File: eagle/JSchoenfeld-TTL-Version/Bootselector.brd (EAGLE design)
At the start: 22 x 64.2 mm, 10 parts, among them IC3 74HC00N, IC4 74HC157N

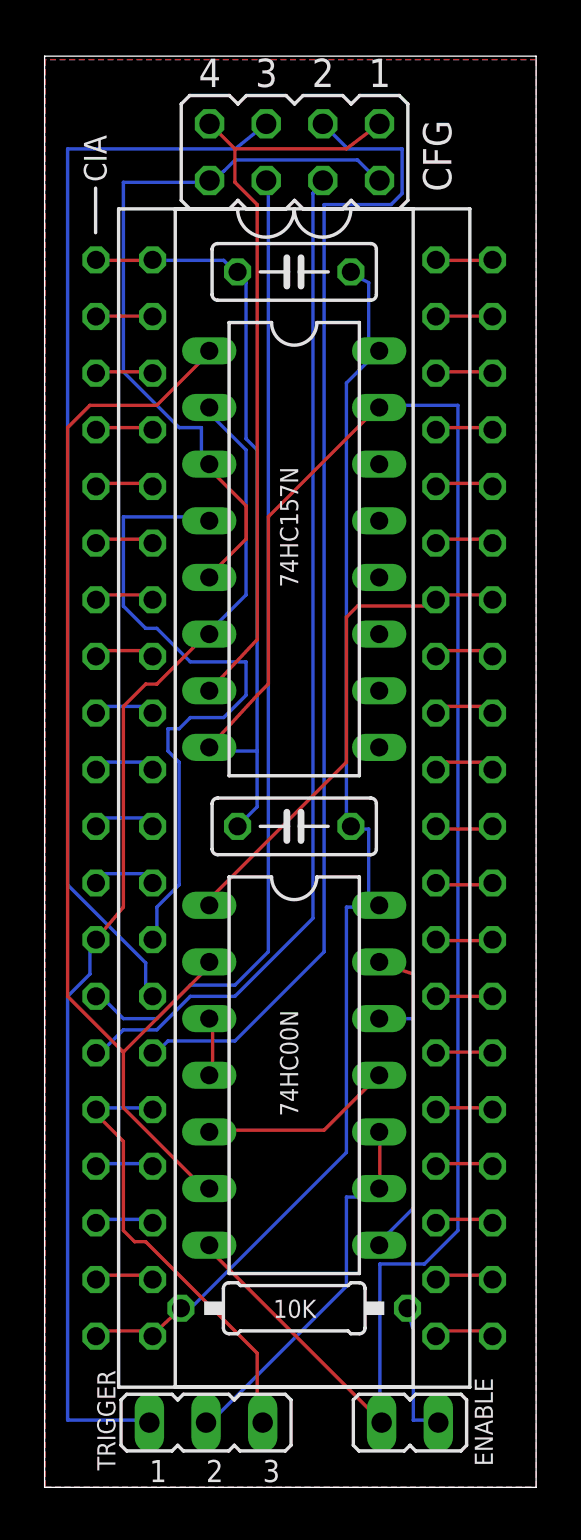
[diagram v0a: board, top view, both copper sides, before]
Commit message: 0.96
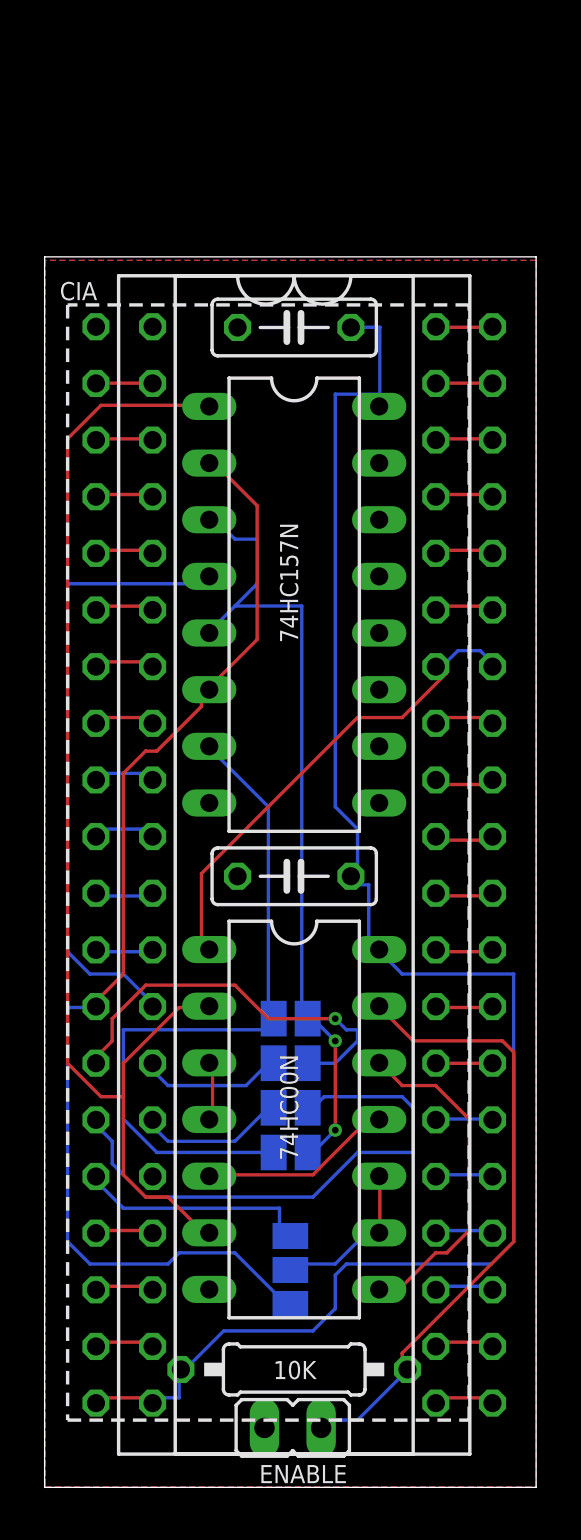
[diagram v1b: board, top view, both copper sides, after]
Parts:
- removed A500: (no value), Amiga:DIP40-6
- removed CFG: (no value), jumper:JP4Q
- added BRD: (no value), Amiga:DIP40-6
- added SJ1, SJ2, SJ3, SJ4: (no value), jumper:SJ
- TRIGGER: value 1-2=KS<2.0 -> (none); device jumper:JP2 -> jumper:SJ_2
- moved TRIGGER 7.82 mm to (11.0, 9.73), flipped to the bottom, turned to 270 degrees
- moved ENABLE 5.26 mm to (11.1, 2.65)
- moved CIA 3.00 mm to (9.89, 27.9)
- moved R1 2.75 mm to (11.2, 5.27)
- moved C1 2.49 mm to (11.2, 52.0)
- moved IC4 2.49 mm to (11.2, 39.6)
- moved C2 2.24 mm to (11.2, 27.4)
- moved IC3 1.98 mm to (11.2, 16.5)
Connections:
- net N$7 renamed TRG
- net N$8 renamed SELENABLE
- net TRIGGER renamed /TRGSEL
- removed net /NEW_SELX: CFG.1, CFG.7, IC4.7
- new net /NEWSELX: IC4.7, SJ1.2, SJ4.2
- new net /SEL3: CIA.16, TRIGGER.1
- net /NEWSEL0: now also BRD.13; no longer A500.13
- net /NEWSEL1: now also BRD.14, SJ2.2; no longer A500.14, CFG.5
- net /NEWSEL2: now also BRD.15, SJ3.2; no longer A500.15, CFG.3
- net /SEL0: now also TRIGGER.3; no longer TRIGGER.1
- net /SEL1: now also SJ2.1; no longer CFG.6
- net /SEL2: now also SJ3.1; no longer CFG.4
- net /SELX: now also SJ1.1, SJ4.1; no longer CFG.2, CFG.8
- net C: now also BRD.40; no longer A500.40
- net CS: now also BRD.23; no longer A500.23
- net D0: now also BRD.26; no longer A500.26
- net D1: now also BRD.27; no longer A500.27
- net D2: now also BRD.28; no longer A500.28
- net D3: now also BRD.29; no longer A500.29
- net D4: now also BRD.30; no longer A500.30
- net D5: now also BRD.31; no longer A500.31
- net D6: now also BRD.32; no longer A500.32
- net D7: now also BRD.33; no longer A500.33
- net E: now also BRD.25; no longer A500.25
- net F: now also BRD.24; no longer A500.24
- net GND: now also BRD.1; no longer A500.1
- net INT: now also BRD.21; no longer A500.21
- net PA0: now also BRD.2; no longer A500.2
- net PA1: now also BRD.3; no longer A500.3
- net PA2: now also BRD.4; no longer A500.4
- net PA3: now also BRD.5; no longer A500.5
- net PA4: now also BRD.6; no longer A500.6
- net PA5: now also BRD.7; no longer A500.7
- net PA6: now also BRD.8; no longer A500.8
- net PA7: now also BRD.9; no longer A500.9
- net PB0: now also BRD.10; no longer A500.10
- net PB1: now also BRD.11; no longer A500.11
- net PB2: now also BRD.12; no longer A500.12
- net PB6: now also BRD.16; no longer A500.16, CIA.16, TRIGGER.3
- net PB7: now also BRD.17; no longer A500.17
- net PC: now also BRD.18; no longer A500.18
- net RESET: now also BRD.34; no longer A500.34
- net RS0: now also BRD.38; no longer A500.38
- net RS1: now also BRD.37; no longer A500.37
- net RS2: now also BRD.36; no longer A500.36
- net RS3: now also BRD.35; no longer A500.35
- net S: now also BRD.39; no longer A500.39
- net TICK: now also BRD.19; no longer A500.19
- net VCC: now also BRD.20; no longer A500.20
- net W: now also BRD.22; no longer A500.22
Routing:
- net GND: track 115.7 -> 0.00 mm
- net /NEWSEL2: track 52.8 -> 6.57 mm
- net /NEWSEL1: track 48.9 -> 6.88 mm
- net /NEW_SELX: track 34.0 -> 0.00 mm
- net /NEWSELX: track 0.00 -> 32.4 mm
- net /SEL1: track 44.0 -> 17.9 mm, vias 0 -> 1
- net /SEL2: track 45.5 -> 24.3 mm
- net PB6: track 20.0 -> 0.00 mm
- net VCC: track 58.0 -> 75.7 mm
- net /SEL3: track 0.00 -> 10.4 mm
- net /TRGSEL: track 17.0 -> 7.35 mm
- net N$2: track 22.9 -> 28.4 mm
- net /SELX: track 33.5 -> 36.8 mm, vias 0 -> 2
- net N$4: track 12.3 -> 15.3 mm
- net SELENABLE: track 50.5 -> 52.9 mm
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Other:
- board size 22 x 64.2 mm -> 22 x 55.2 mm
- board text added: "SEL0 | SEL3"
- board text removed: "A1k"
